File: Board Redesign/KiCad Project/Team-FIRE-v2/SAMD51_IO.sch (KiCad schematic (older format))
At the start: 23 parts

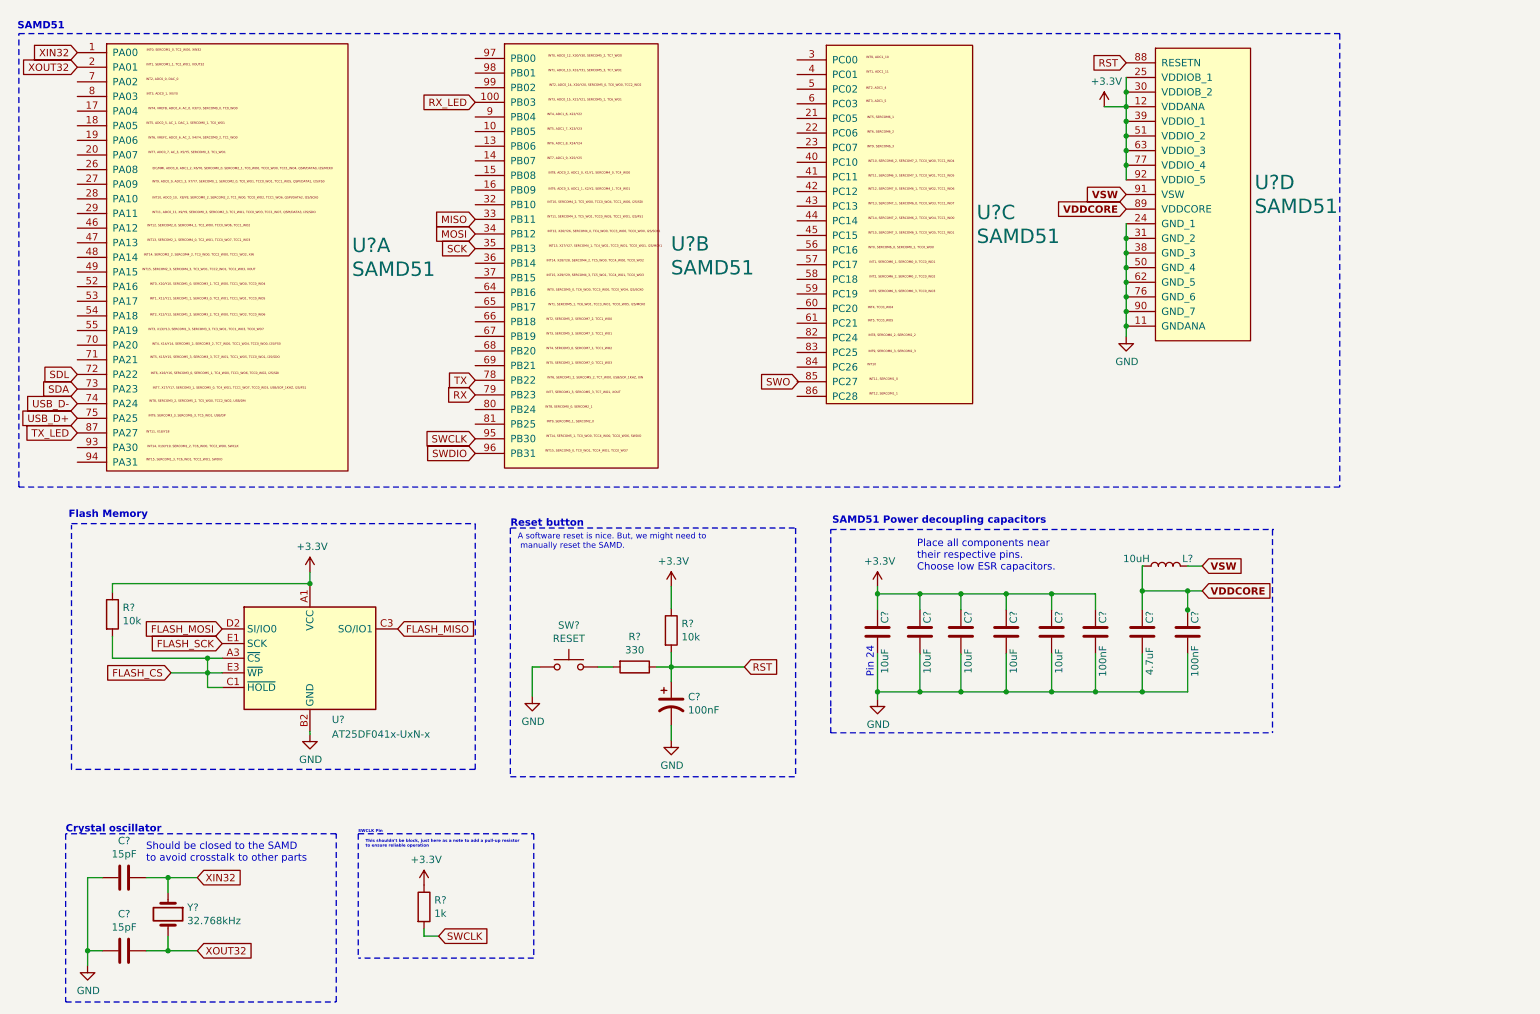
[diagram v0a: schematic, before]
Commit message: Fix connections
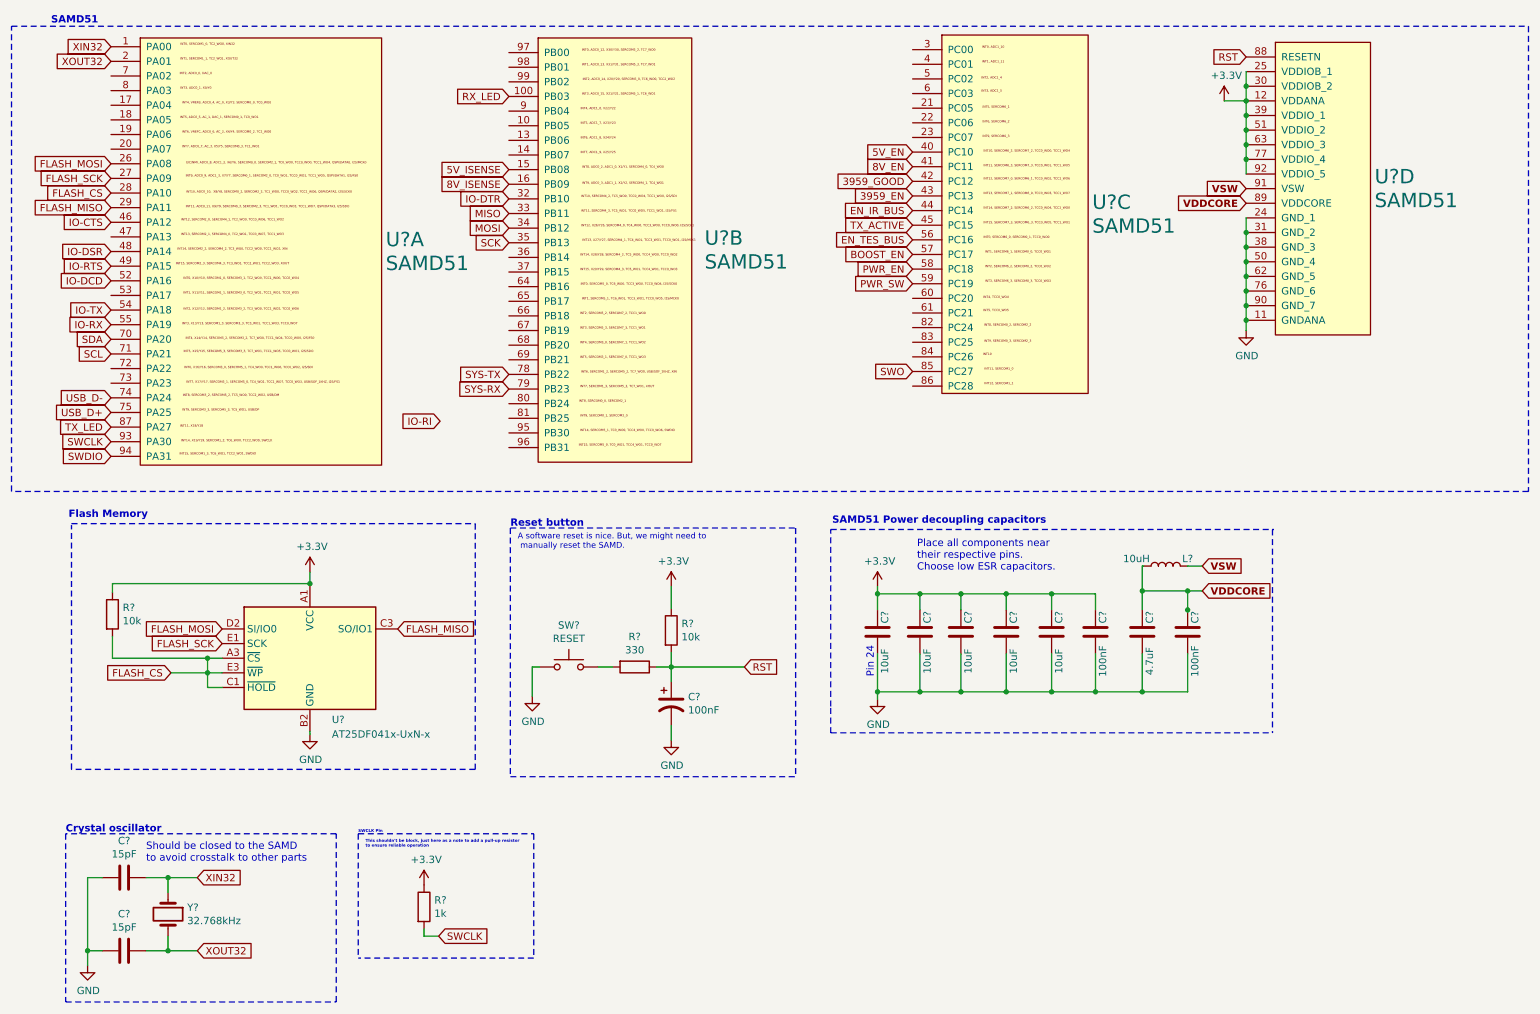
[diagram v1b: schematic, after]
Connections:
- net FLASH_CS: now also U?.28 (PA10)
- net FLASH_MISO: now also U?.29 (PA11)
- net FLASH_MOSI: now also U?.26 (PA08)
- net FLASH_SCK: now also U?.27 (PA09)
- net SDA: now also U?.70 (PA20); no longer U?.73 (PA23)
- net SWCLK: now also U?.93 (PA30); no longer U?.95 (PB30)
- net SWDIO: now also U?.94 (PA31); no longer U?.96 (PB31)
- net SWO: now also U?.85 (PC27)
- net IO-CTS: now reaches U?.46 (PA12)
- net IO-DSR: now reaches U?.48 (PA14)
- net IO-RTS: now reaches U?.49 (PA15)
- net IO-DCD: now reaches U?.52 (PA16)
- net IO-TX: now reaches U?.54 (PA18)
- net IO-RX: now reaches U?.55 (PA19)
- net SCL: now reaches U?.71 (PA21)
- net 5V_ISENSE: now reaches U?.15 (PB08)
- net 8V_ISENSE: now reaches U?.16 (PB09)
- net IO-DTR: now reaches U?.32 (PB10)
- net 5V_EN: now reaches U?.40 (PC10)
- net 8V_EN: now reaches U?.41 (PC11)
- net 3959_GOOD: now reaches U?.42 (PC12)
- net 3959_EN: now reaches U?.43 (PC13)
- net EN_IR_BUS: now reaches U?.44 (PC14)
- net TX_ACTIVE: now reaches U?.45 (PC15)
- net EN_TES_BUS: now reaches U?.56 (PC16)
- net BOOST_EN: now reaches U?.57 (PC17)
- net PWR_EN: now reaches U?.58 (PC18)
- net PWR_SW: now reaches U?.59 (PC19)
- net RX renamed SYS-RX
- net SDL: no longer names the net of U?.72 (PA22)
- net TX renamed SYS-TX
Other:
- moved on the sheet: U?A, U?B, U?C, U?D
